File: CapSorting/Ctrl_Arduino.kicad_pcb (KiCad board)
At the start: 2 copper layers, 0 parts

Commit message: Android　シール用追加
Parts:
- added A12: Arduino_UNO_R3, Module:Arduino_UNO_R2, B.Cu at (100.0, 100.0)
- added C1: 0.22u, Resistor_SMD:R_0402_1005Metric, F.Cu at (89.4, 119.7)
- added C12: 0.22u, Resistor_SMD:R_0402_1005Metric, F.Cu at (103.3, 119.7)
- added C13: 0.22u, Resistor_SMD:R_0402_1005Metric, F.Cu at (117.2, 120.0)
- added C14: 0.22u, Resistor_SMD:R_0402_1005Metric, F.Cu at (99.6, 119.7)
- added C15: 0.22u, Resistor_SMD:R_0402_1005Metric, F.Cu at (113.2, 120.0)
- added C2: 0.22u, Resistor_SMD:R_0402_1005Metric, F.Cu at (85.9, 119.6)
- added D1: RB060M-60TR, Diode_SMD:D_1206_3216Metric, F.Cu at (90.8, 115.2)
- added D12: RB060M-60TR, Diode_SMD:D_1206_3216Metric, F.Cu at (101.1, 115.3)
- added D13: RB060M-60TR, Diode_SMD:D_1206_3216Metric, F.Cu at (104.8, 115.3)
- added D14: RB060M-60TR, Diode_SMD:D_1206_3216Metric, F.Cu at (114.7, 115.3)
- added D15: RB060M-60TR, Diode_SMD:D_1206_3216Metric, F.Cu at (118.7, 115.3)
- added D2: RB060M-60TR, Diode_SMD:D_1206_3216Metric, F.Cu at (87.3, 115.2)
- added J1: Conn_01x10, JST:S10B-XH-A, F.Cu at (102.5, 108.0)
- added L12: 6.8uH(74404042068), Ctrl_Arduino:INDPM4040X180N, F.Cu at (117.6, 106.3)
- added R1: 1k, Resistor_SMD:R_0603_1608Metric, F.Cu at (90.8, 119.4)
- added R12: 1k, Resistor_SMD:R_0603_1608Metric, F.Cu at (108.3, 126.7)
- added R13: 1k, Resistor_SMD:R_0603_1608Metric, F.Cu at (94.5, 126.6)
- added R14: 1k, Resistor_SMD:R_0603_1608Metric, F.Cu at (114.7, 119.7)
- added R15: 1k, Resistor_SMD:R_0603_1608Metric, F.Cu at (101.1, 119.4)
- added R16: 1k, Resistor_SMD:R_0603_1608Metric, F.Cu at (118.7, 119.7)
- added R17: 1k, Resistor_SMD:R_0603_1608Metric, F.Cu at (104.8, 119.4)
- added R2: 1k, Resistor_SMD:R_0603_1608Metric, F.Cu at (87.3, 119.3)
- added R3: 1k, Resistor_SMD:R_0603_1608Metric, F.Cu at (80.6, 126.8)
- added U1: TLP785, Package_DIP:DIP-4_W7.62mm, F.Cu at (108.4, 123.7)
- added U13: TLP785, Package_DIP:DIP-4_W7.62mm, F.Cu at (94.5, 123.7)
- added U2: TLP785, Package_DIP:DIP-4_W7.62mm, F.Cu at (80.6, 123.8)
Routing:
- net Net-(A12-Pad20): track 0.00 -> 1.50 mm
- added copper zone on B.Cu, net GND
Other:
- board outline added: 54 x 50.7 mm

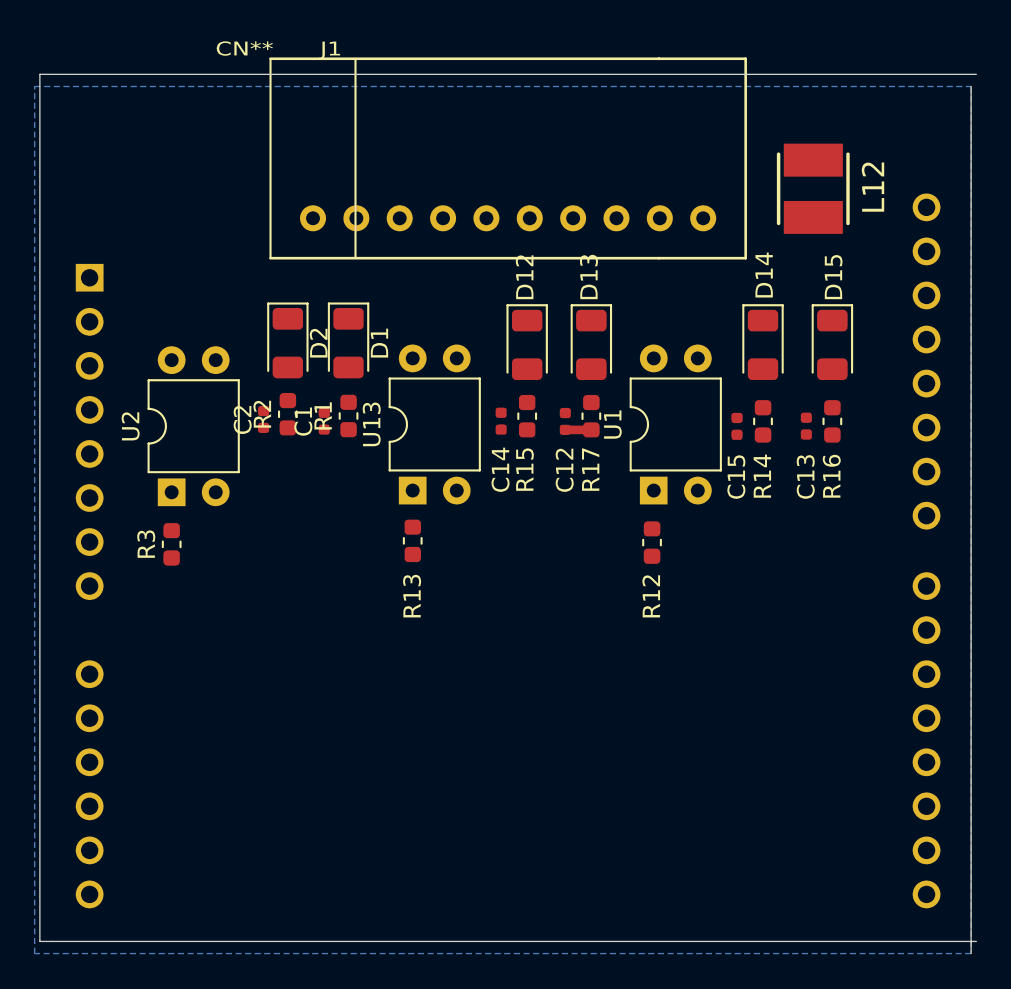
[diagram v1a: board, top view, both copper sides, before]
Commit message: no message
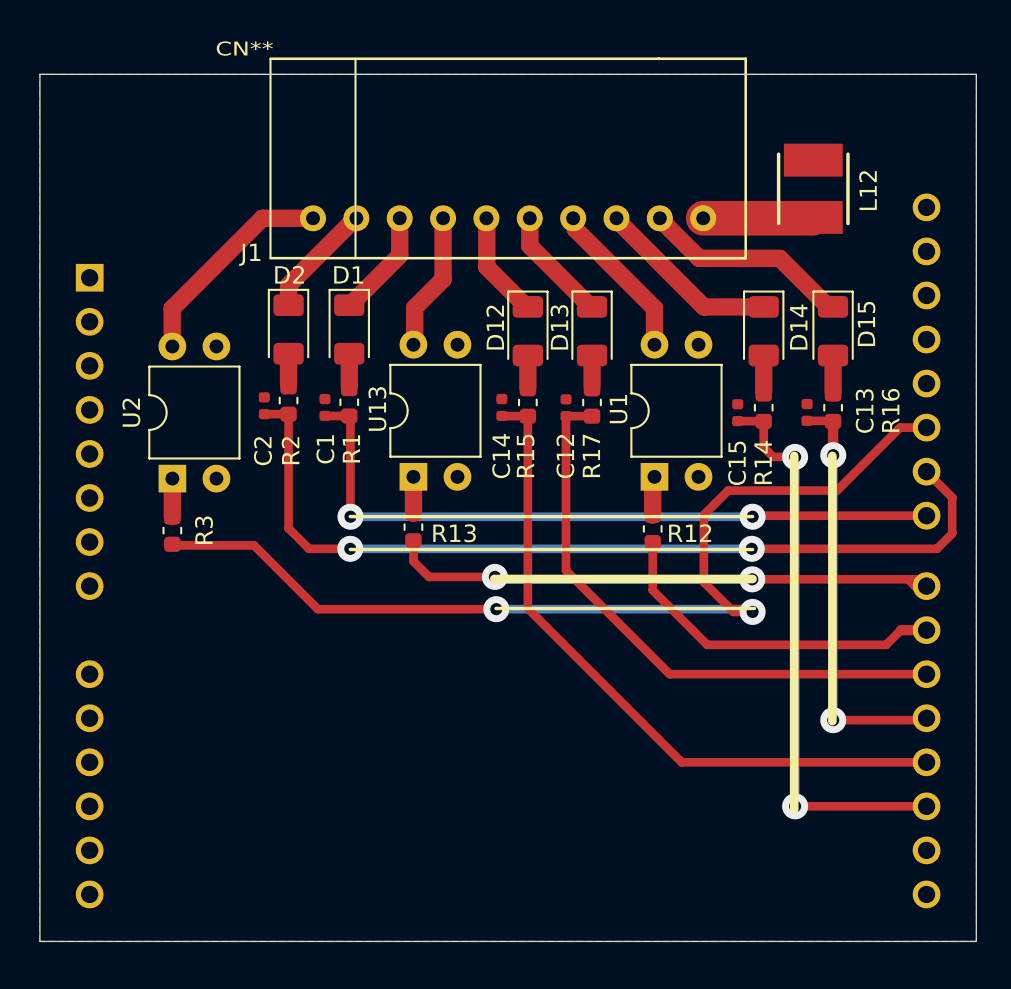
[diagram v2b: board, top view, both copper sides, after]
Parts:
- moved C12 0.79 mm to (103.3, 118.9)
- moved C14 0.79 mm to (99.6, 118.9)
- moved D1 0.79 mm to (90.8, 114.4)
- moved D2 0.79 mm to (87.3, 114.4)
- moved R1 0.79 mm to (90.8, 118.6)
- moved R12 0.79 mm to (108.3, 125.9)
- moved U13 0.79 mm to (94.5, 122.9)
- moved C1 0.79 mm to (89.4, 118.9)
- moved C13 0.79 mm to (117.2, 119.2)
- moved C15 0.79 mm to (113.2, 119.2)
- moved R14 0.79 mm to (114.7, 118.9)
- moved R16 0.79 mm to (118.7, 118.9)
- moved U1 0.79 mm to (108.4, 122.9)
- moved D12 0.79 mm to (101.1, 114.5)
- moved D13 0.79 mm to (104.8, 114.5)
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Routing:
- net Net-(A12-Pad25): track 0.00 -> 58.6 mm, vias 0 -> 2
- net Net-(A12-Pad24): track 0.00 -> 51.2 mm, vias 0 -> 2
- net Net-(A12-Pad23): track 0.00 -> 40.3 mm, vias 0 -> 2
- net Net-(A12-Pad18): track 0.00 -> 39.3 mm
- net Net-(A12-Pad17): track 0.40 -> 33.1 mm, vias 0 -> 2
- net Net-(A12-Pad22): track 0.00 -> 32.5 mm, vias 0 -> 2
- net Net-(A12-Pad20): track 1.50 -> 33.7 mm
- net Net-(A12-Pad19): track 0.00 -> 24.1 mm, vias 0 -> 2
- net Net-(A12-Pad21): track 0.00 -> 20.2 mm
- net AIR1_Y005: track 0.00 -> 12.4 mm
- net PassSensor_Area2: track 0.00 -> 11.7 mm
- net PE_Camera_B17: track 0.00 -> 10.6 mm
- net AIR2_Y006: track 0.00 -> 9.11 mm
- net AIR3_Y012: track 0.00 -> 7.93 mm
- net PassSensor_Area1: track 0.00 -> 6.61 mm
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- added copper zone on F.Cu, net GND
- removed copper zone on B.Cu, net GND
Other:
- board size 54 x 50.7 mm -> 54 x 50 mm
